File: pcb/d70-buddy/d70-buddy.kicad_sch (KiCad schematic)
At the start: 29 parts, among them SW1 SW_SPDT, SW2 SW_Push_LED, U1 TLV61046ADB, U2 TLV70228_SOT23-5

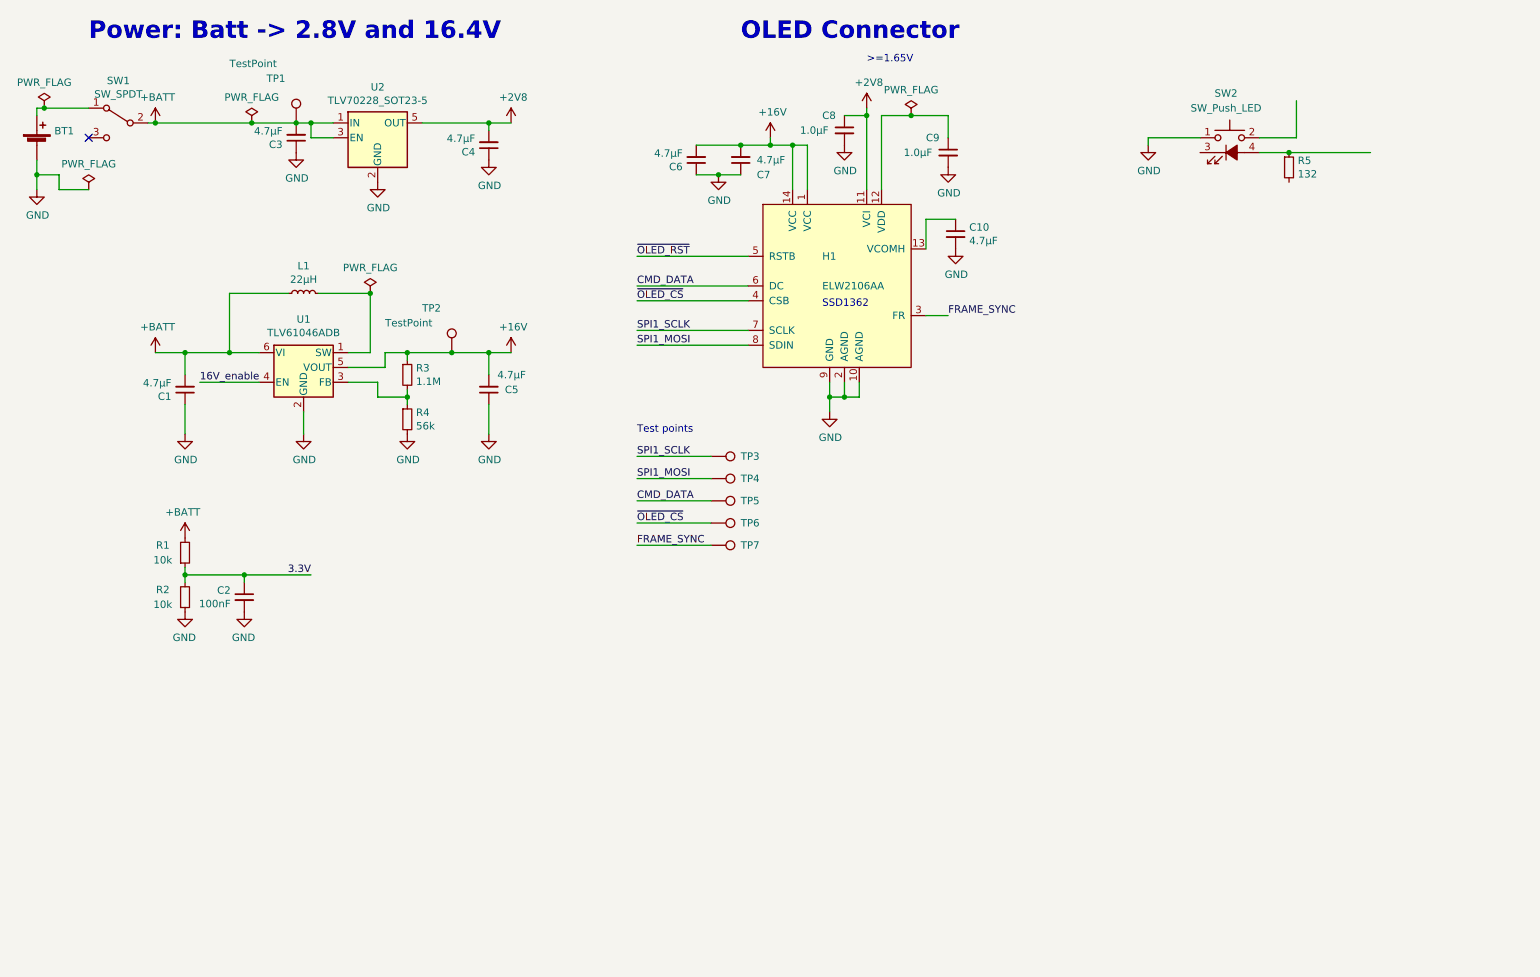
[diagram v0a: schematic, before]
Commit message: more pcb stuff
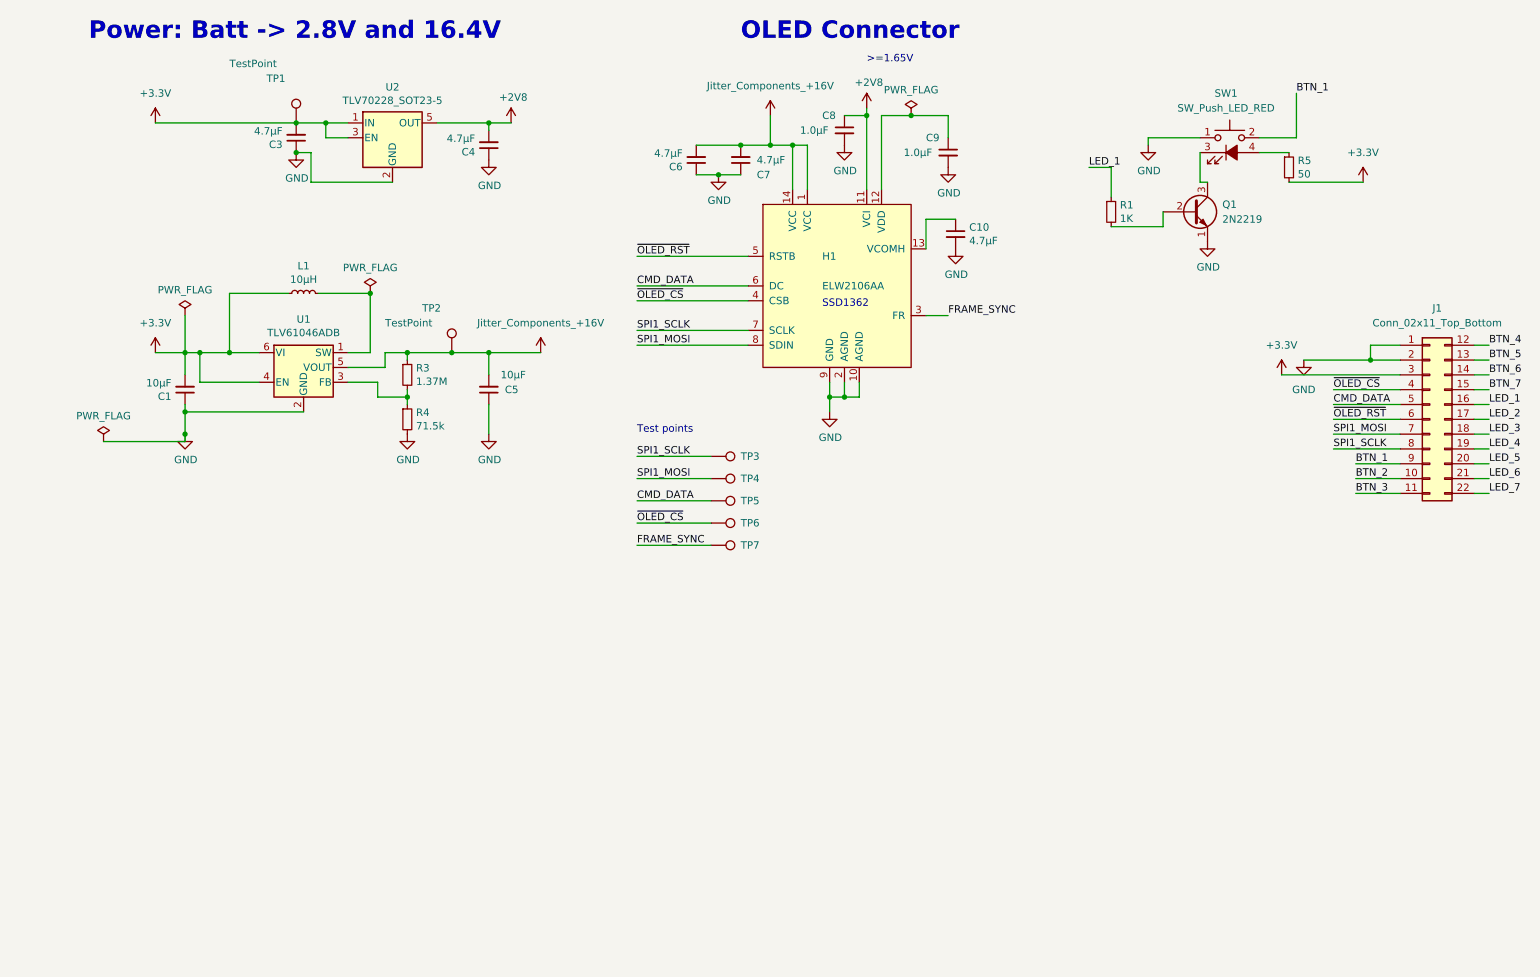
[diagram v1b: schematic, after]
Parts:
- removed BT1: Battery_Cell, Jitter_Footprints:BatteryHolder_Keystone_1043(p)_1x18650, symbol Device:Battery_Cell
- removed C2: 100nF, Capacitor_SMD:C_0402_1005Metric, symbol Device:C_Small
- removed R2: 10k, Resistor_SMD:R_0402_1005Metric, symbol Device:R_Small
- removed SW1: SW_SPDT, Jitter_Footprints:slide_switch_09.03201.02, symbol Switch:SW_SPDT
- added J1: Conn_02x11_Top_Bottom, Connector_PinHeader_2.54mm:PinHeader_2x11_P2.54mm_Vertical, symbol Connector_Generic:Conn_02x11_Top_Bottom
- added Q1: 2N2219, Package_TO_SOT_SMD:TSOT-23, symbol Transistor_BJT:2N2219
- C1, C5: value 4.7µF -> 10µF
- H1: symbol Jitter_Components:ELW2106AA -> serial-logger-prototype-cache:Jitter_Components_ELW2106AA
- L1: value 22µH -> 10µH
- R1: value 10k -> 1K
- R3: value 1.1M -> 1.37M
- R4: value 56k -> 71.5k
- R5: value 132 -> 50
- SW1: renamed from SW2; value SW_Push_LED -> SW_Push_LED_RED; footprint (none) -> lib:SW_PUSH_LED_6mm_H7.3mm; Spice_Lib_File (none) -> C:\workspace\KiCad-Spice-Library\Models\Diode\led.lib; Spice_Model (none) -> LED_GENERAL; Spice_Netlist_Enabled (none) -> Y; Spice_Primitive (none) -> D
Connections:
- net 16V_enable is gone; now on net +3V3: U1.4 (EN)
- net CMD_DATA: now also J1.5 (Pin_5)
- net GND: now also J1.1 (Pin_1), J1.2 (Pin_2), Q1.1 (E)
- net SPI1_MOSI: now also J1.7 (Pin_7)
- net SPI1_SCLK: now also J1.8 (Pin_8)
- net ~{OLED_CS}: now also J1.4 (Pin_4)
- net ~{OLED_RST}: now also J1.6 (Pin_6)
- net +3V3: now reaches R5.2
- net +3V3: now also C1.2, C3.2, L1.1, TP1.1, U1.6 (VI), U2.1 (IN), U2.3 (EN), J1.3 (Pin_3)
- net BTN_1: now reaches SW1.2
- net BTN_1: now also J1.9 (Pin_9)
- net at SW1.3 (K): now also Q1.3 (C)
- removed net +BATT: C1.2, C3.2, L1.1, R1.2, TP1.1, U1.6 (VI), U2.1 (IN), U2.3 (EN)
- net 3.3V renamed LED_1
- net LED_1: now also J1.16 (Pin_16)
- new net: Q1.2 (B), R1.2
- new net BTN_2: J1.10 (Pin_10)
- new net BTN_3: J1.11 (Pin_11)
- new net BTN_4: J1.12 (Pin_12)
- new net BTN_5: J1.13 (Pin_13)
- new net BTN_6: J1.14 (Pin_14)
- new net BTN_7: J1.15 (Pin_15)
- new net LED_2: J1.17 (Pin_17)
- new net LED_3: J1.18 (Pin_18)
- new net LED_4: J1.19 (Pin_19)
- new net LED_5: J1.20 (Pin_20)
- new net LED_6: J1.21 (Pin_21)
- new net LED_7: J1.22 (Pin_22)
- no-connect marks 1 -> 0
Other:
- moved on the sheet: U2

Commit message: wip
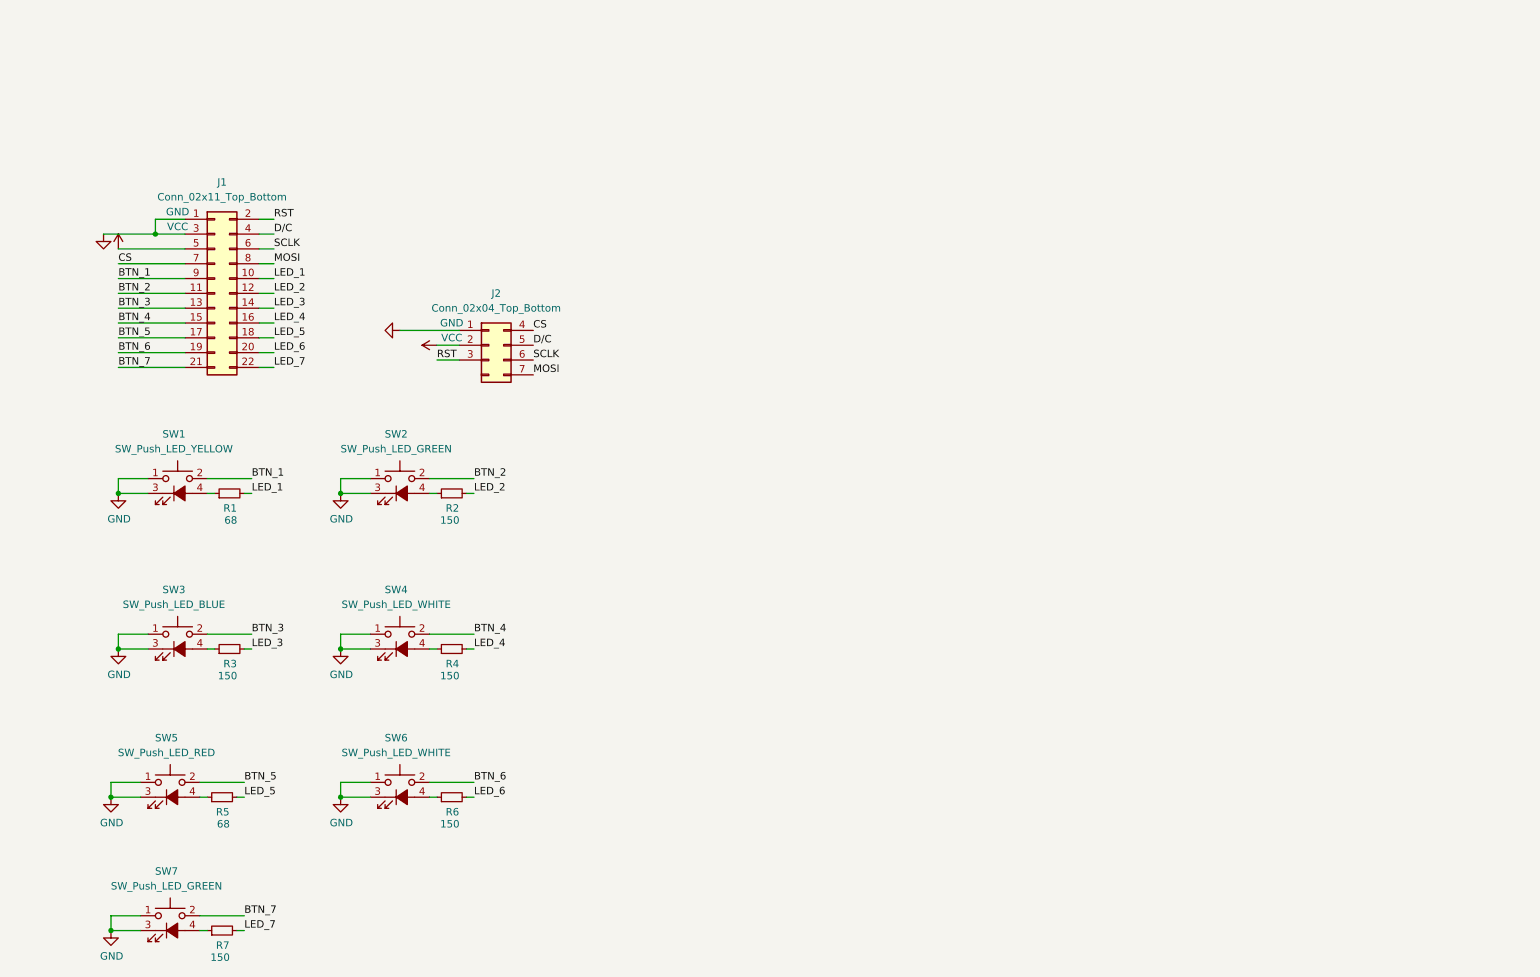
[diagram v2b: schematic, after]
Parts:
- removed C1, C5: 10µF, Capacitor_SMD:C_0805_2012Metric, symbol Device:C_Small
- removed C10, C3, C4, C6, C7: 4.7µF, Capacitor_SMD:C_0805_2012Metric, symbol Device:C_Small
- removed C8, C9: 1.0µF, Capacitor_SMD:C_0603_1608Metric, symbol Device:C_Small
- removed H1: ELW2106AA, lib:MOLEX_503480-1400, symbol serial-logger-prototype-cache:Jitter_Components_ELW2106AA
- removed L1: 10µH, Inductor_SMD:L_1812_4532Metric, symbol Device:L_Small
- removed Q1: 2N2219, Package_TO_SOT_SMD:TSOT-23, symbol Transistor_BJT:2N2219
- removed TP1, TP2: TestPoint, TestPoint:TestPoint_Pad_D1.5mm, symbol Connector:TestPoint
- removed TP3, TP4, TP5, TP6, TP7: TestPoint, TestPoint:TestPoint_Pad_D1.0mm, symbol Connector:TestPoint
- removed U1: TLV61046ADB, Package_TO_SOT_SMD:SOT-23-6, symbol Regulator_Switching:TLV61046ADB
- removed U2: TLV70228_SOT23-5, Package_TO_SOT_SMD:SOT-23-5, symbol Regulator_Linear:TLV70228_SOT23-5
- added J2: Conn_02x04_Top_Bottom, lib:ELW2106AA, symbol Connector_Generic:Conn_02x04_Top_Bottom
- added R2, R6, R7: 150, Resistor_SMD:R_0402_1005Metric, symbol Device:R_Small
- added SW2, SW7: SW_Push_LED_GREEN, lib:SW_PUSH_LED_6mm_H7.3mm, symbol Switch:SW_Push_LED
- added SW3: SW_Push_LED_BLUE, lib:SW_PUSH_LED_6mm_H7.3mm, symbol Switch:SW_Push_LED
- added SW4, SW6: SW_Push_LED_WHITE, lib:SW_PUSH_LED_6mm_H7.3mm, symbol Switch:SW_Push_LED
- added SW5: SW_Push_LED_RED, lib:SW_PUSH_LED_6mm_H7.3mm, symbol Switch:SW_Push_LED
- J1: symbol Connector_Generic:Conn_02x11_Top_Bottom -> Connector_Generic:Conn_02x11_Odd_Even
- R1: value 1K -> 68
- R3: value 1.37M -> 150
- R4: value 71.5k -> 150
- R5: value 50 -> 68
- SW1: value SW_Push_LED_RED -> SW_Push_LED_YELLOW
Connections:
- net BTN_2: now also J1.11 (Pin_11), SW2.2; no longer J1.10 (Pin_10)
- net BTN_3: now also J1.13 (Pin_13), SW3.2; no longer J1.11 (Pin_11)
- net BTN_4: now also J1.15 (Pin_15), SW4.2; no longer J1.12 (Pin_12)
- net BTN_5: now also J1.17 (Pin_17), SW5.2; no longer J1.13 (Pin_13)
- net BTN_6: now also J1.19 (Pin_19), SW6.2; no longer J1.14 (Pin_14)
- net BTN_7: now also J1.21 (Pin_21), SW7.2; no longer J1.15 (Pin_15)
- net GND: now also J1.3 (Pin_3), SW1.3 (K), J2.1 (Pin_1), SW2.1, SW2.3 (K), SW3.1, SW3.3 (K), SW4.1, SW4.3 (K), SW5.1, SW5.3 (K), SW6.1, SW6.3 (K), SW7.1, SW7.3 (K); no longer J1.2 (Pin_2), R4.2
- net LED_1: now also J1.10 (Pin_10), R1.2; no longer J1.16 (Pin_16), R1.1
- net LED_2: now also J1.12 (Pin_12), R2.2; no longer J1.17 (Pin_17)
- net LED_3: now also J1.14 (Pin_14), R3.2; no longer J1.18 (Pin_18)
- net LED_4: now also J1.16 (Pin_16), R4.2; no longer J1.19 (Pin_19)
- net LED_5: now also J1.18 (Pin_18), R5.2; no longer J1.20 (Pin_20)
- net LED_6: now also J1.20 (Pin_20), R6.2; no longer J1.21 (Pin_21)
- net LED_7: now also R7.2
- net at R4.1: now also SW4.4 (A); no longer R3.2
- net at SW1.4 (A): now also R1.1; no longer R5.1
- net +16V: no longer names the net of R3.1
- net +16V: now also SW3.4 (A)
- removed net +3V3: J1.3 (Pin_3), R5.2
- net CMD_DATA renamed VCC
- net VCC: now also J2.2 (Pin_2)
- net SPI1_MOSI renamed CS
- net CS: now also J2.4 (Pin_4)
- net SPI1_SCLK renamed MOSI
- net MOSI: now also J2.7 (Pin_7)
- net ~{OLED_CS} renamed D/C
- net D/C: now also J2.5 (Pin_5)
- net ~{OLED_RST} renamed SCLK
- net SCLK: now also J2.6 (Pin_6)
- new net: R6.1, SW6.4 (A)
- new net: R2.1, SW2.4 (A)
- new net: R5.1, SW5.4 (A)
- new net: R7.1, SW7.4 (A)
- new net RST: J1.2 (Pin_2), J2.3 (Pin_3)
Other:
- note removed: ">=1.65V"
- note removed: "OLED Connector"
- note removed: "Power: Batt -> 2.8V and 16.4V"
- note removed: "SSD1362"
- note removed: "Test points"
- moved on the sheet: J1

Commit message: Wip
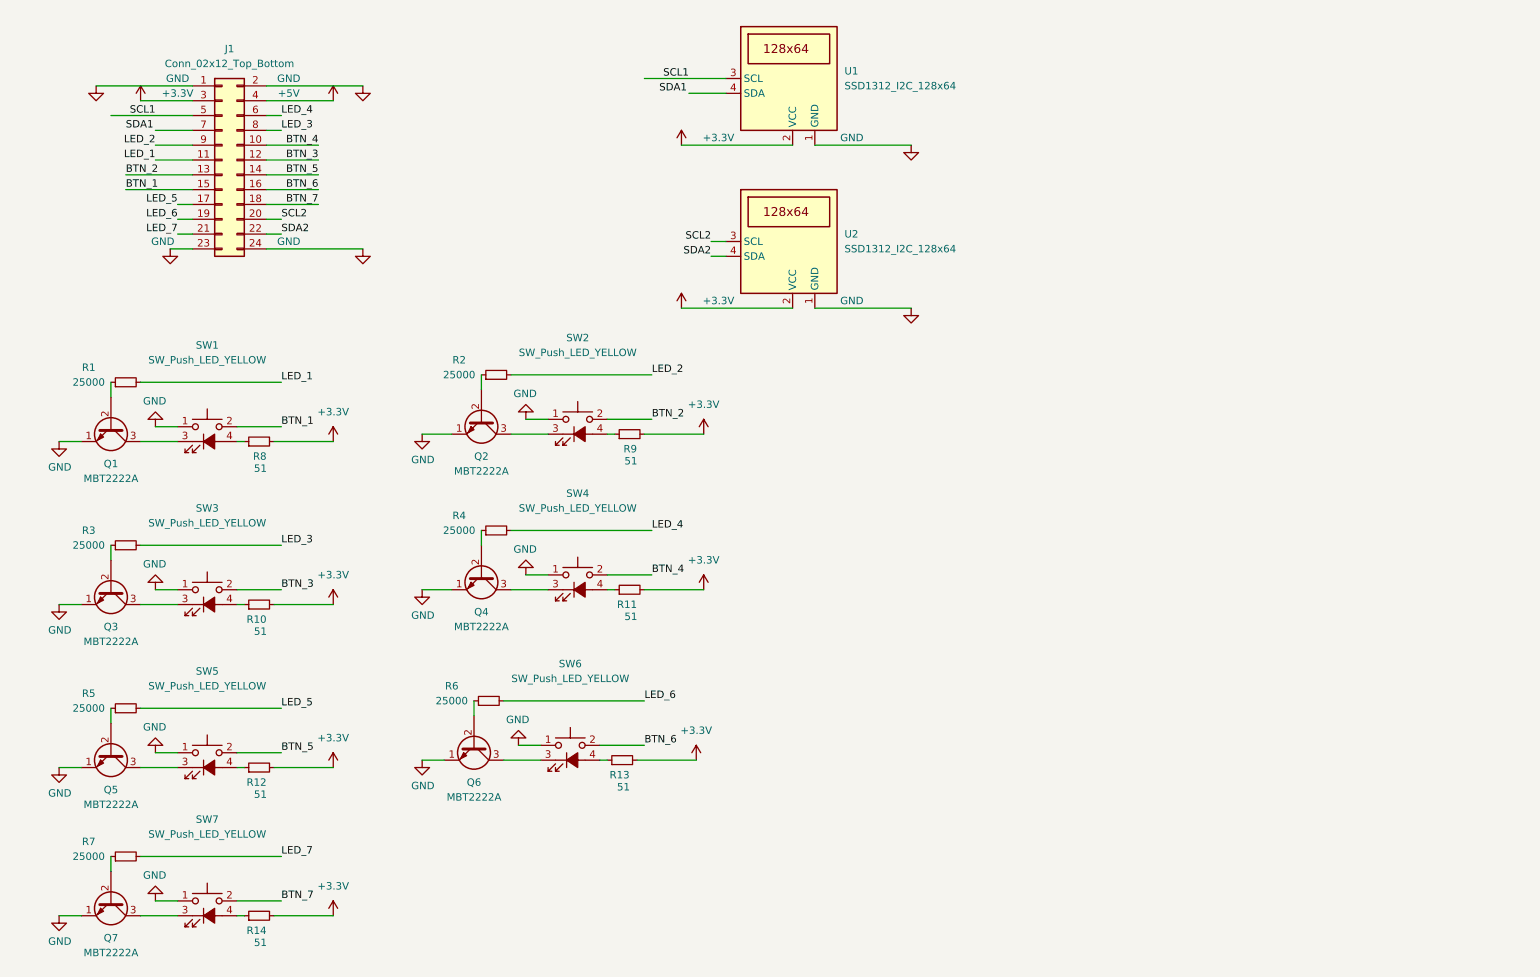
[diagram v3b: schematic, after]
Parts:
- removed J2: Conn_02x04_Top_Bottom, lib:ELW2106AA, symbol Connector_Generic:Conn_02x04_Top_Bottom
- added Q1, Q2, Q3, Q4, Q5, Q6, Q7: MBT2222A, Package_TO_SOT_SMD:SOT-23, symbol Transistor_BJT:2N2219
- added R10, R11, R12, R13, R14, R8, R9: 51, Resistor_SMD:R_0402_1005Metric, symbol Device:R_Small
- added U1, U2: SSD1312_I2C_128x64, OLED SSD1312 KiCAD:OLED_SSD1312_I2C_0.96_No_Mounting_Holes, symbol OLED_SSD1312_I2C:SSD1312_I2C_128x64
- J1: value Conn_02x11_Top_Bottom -> Conn_02x12_Top_Bottom; footprint Connector_PinHeader_2.54mm:PinHeader_2x11_P2.54mm_Vertical -> Connector_PinHeader_2.54mm:PinHeader_2x12_P2.54mm_Vertical; symbol Connector_Generic:Conn_02x11_Odd_Even -> Connector_Generic:Conn_02x12_Odd_Even
- R1, R5: value 68 -> 25000; footprint Resistor_SMD:R_0402_1005Metric -> Resistor_SMD:R_0201_0603Metric
- R2, R3, R4, R6, R7: value 150 -> 25000; footprint Resistor_SMD:R_0402_1005Metric -> Resistor_SMD:R_0201_0603Metric
- SW2, SW7: value SW_Push_LED_GREEN -> SW_Push_LED_YELLOW
- SW3: value SW_Push_LED_BLUE -> SW_Push_LED_YELLOW
- SW4, SW6: value SW_Push_LED_WHITE -> SW_Push_LED_YELLOW
- SW5: value SW_Push_LED_RED -> SW_Push_LED_YELLOW
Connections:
- net MOSI is gone; now on net LED_3: J1.8 (Pin_8)
- net RST is gone; now on net GND: J1.2 (Pin_2)
- net SCLK is gone; now on net LED_4: J1.6 (Pin_6)
- net BTN_1: now also J1.15 (Pin_15); no longer J1.9 (Pin_9)
- net BTN_2: now also J1.13 (Pin_13); no longer J1.11 (Pin_11)
- net BTN_3: now also J1.12 (Pin_12); no longer J1.13 (Pin_13)
- net BTN_4: now also J1.10 (Pin_10); no longer J1.15 (Pin_15)
- net BTN_5: now also J1.14 (Pin_14); no longer J1.17 (Pin_17)
- net BTN_6: now also J1.16 (Pin_16); no longer J1.19 (Pin_19)
- net BTN_7: now also J1.18 (Pin_18); no longer J1.21 (Pin_21)
- net GND: now also J1.23 (Pin_23), J1.24 (Pin_24), Q1.1 (E), Q2.1 (E), Q3.1 (E), Q4.1 (E), Q5.1 (E), Q6.1 (E), Q7.1 (E), U1.1 (GND), U2.1 (GND); no longer J1.3 (Pin_3), SW1.3 (K), SW2.3 (K), SW3.3 (K), SW4.3 (K), SW5.3 (K), SW6.3 (K), SW7.3 (K)
- net LED_1: now also J1.11 (Pin_11); no longer J1.10 (Pin_10)
- net LED_2: now also J1.9 (Pin_9); no longer J1.12 (Pin_12)
- net LED_3: no longer J1.14 (Pin_14)
- net LED_4: no longer J1.16 (Pin_16)
- net LED_5: now also J1.17 (Pin_17); no longer J1.18 (Pin_18)
- net LED_6: now also J1.19 (Pin_19); no longer J1.20 (Pin_20)
- net LED_7: now also J1.21 (Pin_21); no longer J1.22 (Pin_22)
- net at SW1.4 (A): now also R8.1; no longer R1.1
- net at SW4.4 (A): now also R11.1; no longer R4.1
- net at SW6.4 (A): now also R13.1; no longer R6.1
- net at R2.1: now also Q2.2 (B); no longer SW2.4 (A)
- net at R3.1: now also Q3.2 (B); no longer SW3.4 (A)
- net at SW5.4 (A): now also R12.1; no longer R5.1
- net at R7.1: now also Q7.2 (B); no longer SW7.4 (A)
- net CS: no longer names the net of J1.7 (Pin_7)
- net D/C renamed +5V
- net VCC renamed SCL1
- net SCL1: now also U1.3 (SCL)
- new net: Q4.3 (C), SW4.3 (K)
- new net: Q3.3 (C), SW3.3 (K)
- new net: Q1.3 (C), SW1.3 (K)
- new net: Q6.3 (C), SW6.3 (K)
- new net: R14.1, SW7.4 (A)
- new net: R10.1, SW3.4 (A)
- new net: Q1.2 (B), R1.1
- new net: Q2.3 (C), SW2.3 (K)
- new net: Q6.2 (B), R6.1
- new net: R9.1, SW2.4 (A)
- new net: Q7.3 (C), SW7.3 (K)
- new net: Q5.3 (C), SW5.3 (K)
- new net: Q5.2 (B), R5.1
- new net: Q4.2 (B), R4.1
- new net +3V3: J1.3 (Pin_3), R10.2, R11.2, R12.2, R13.2, R14.2, R8.2, R9.2, U1.2 (VCC), U2.2 (VCC)
- new net SCL2: J1.20 (Pin_20), U2.3 (SCL)
- new net SDA2: J1.22 (Pin_22), U2.4 (SDA)
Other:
- moved on the sheet: SW1
